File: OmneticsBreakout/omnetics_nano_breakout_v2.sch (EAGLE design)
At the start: 2 parts

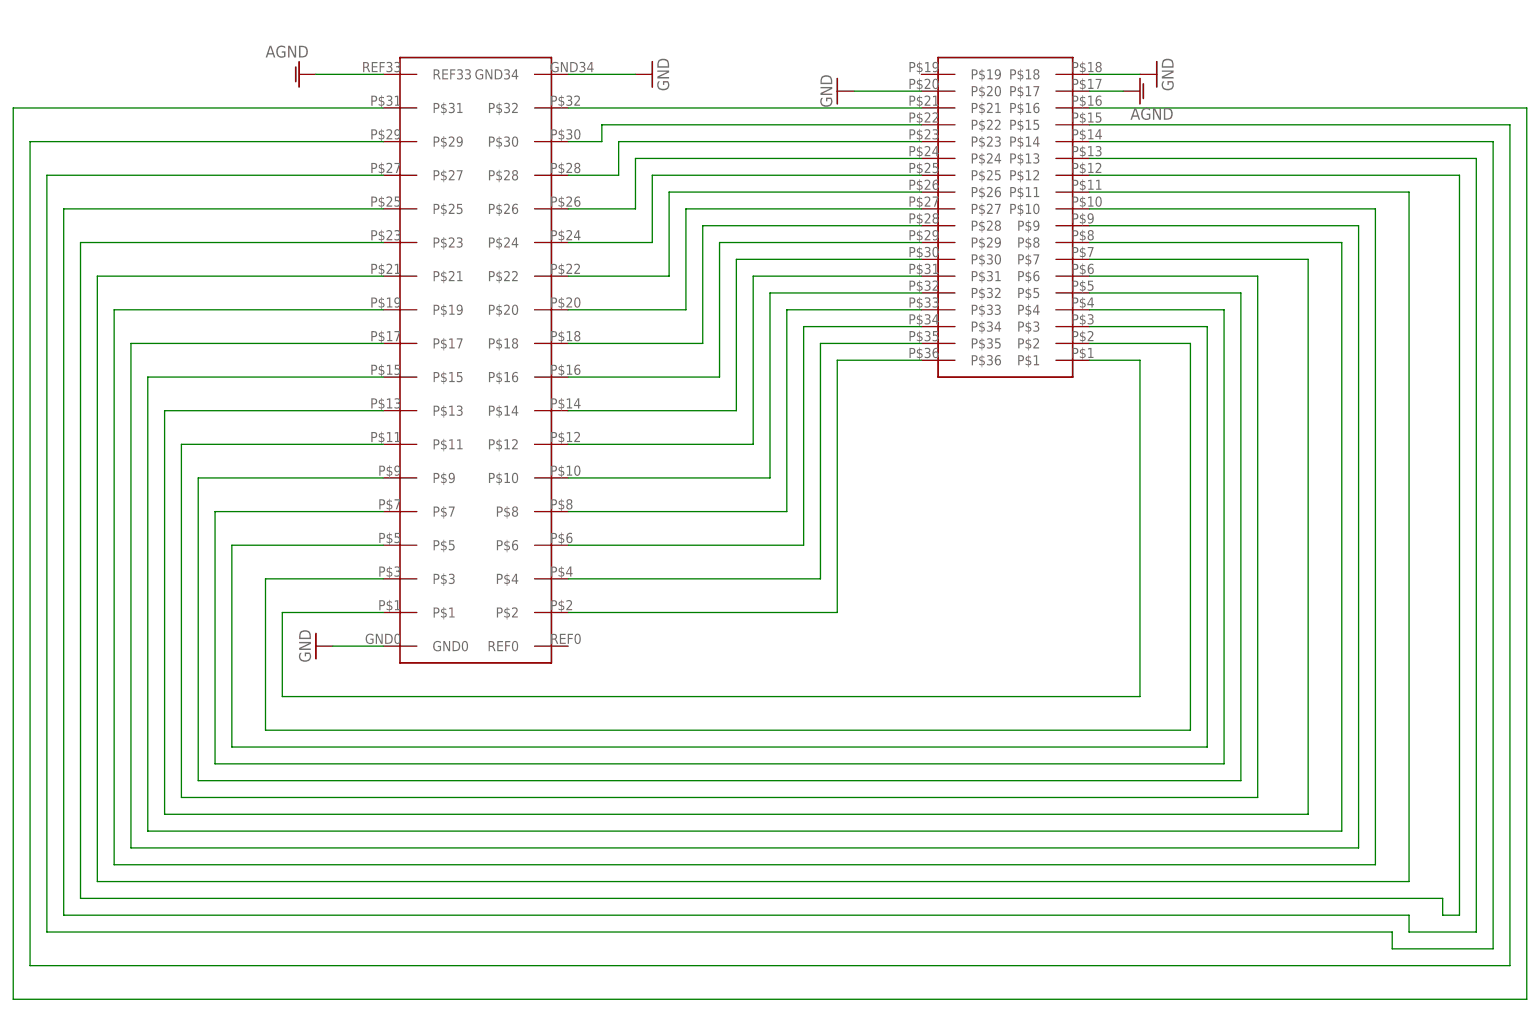
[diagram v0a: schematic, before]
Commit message: omentics breakout board
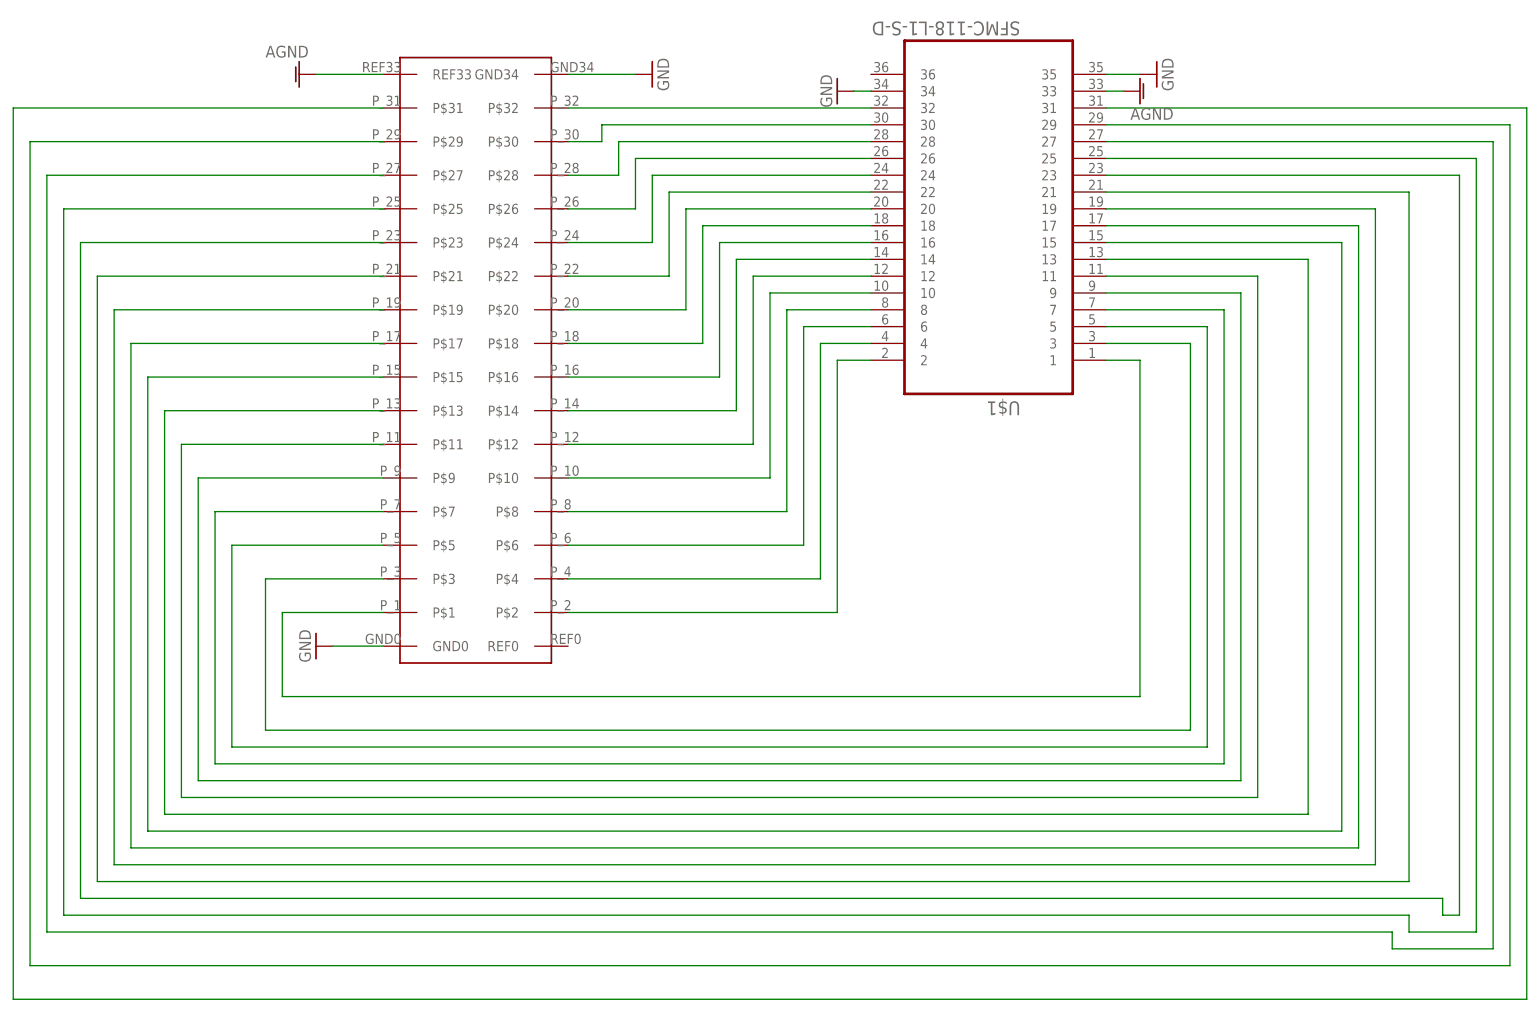
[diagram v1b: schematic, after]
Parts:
- U$1: value FSTH-118-01-F-D -> SFMC-118-L1-S-D; device Sombeck_lib:FSTH-118-01-F-D -> tuckerLib:SFMC-118-L1-S-D
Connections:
- net AGND: now also U$1.33; no longer U$1.P$17
- net GND: now also U$1.34, U$1.35; no longer U$1.P$18, U$1.P$20
- net N$1: now also U$1.1; no longer U$1.P$1
- net N$10: now also U$1.18; no longer U$1.P$28
- net N$11: now also U$1.20; no longer U$1.P$27
- net N$12: now also U$1.22; no longer U$1.P$26
- net N$13: now also U$1.24; no longer U$1.P$25
- net N$14: now also U$1.26; no longer U$1.P$24
- net N$15: now also U$1.28; no longer U$1.P$23
- net N$16: now also U$1.30; no longer U$1.P$22
- net N$17: now also U$1.32; no longer U$1.P$21
- net N$18: now also U$1.3; no longer U$1.P$2
- net N$19: now also U$1.5; no longer U$1.P$3
- net N$2: now also U$1.2; no longer U$1.P$36
- net N$20: now also U$1.7; no longer U$1.P$4
- net N$21: now also U$1.9; no longer U$1.P$5
- net N$22: now also U$1.11; no longer U$1.P$6
- net N$23: now also U$1.13; no longer U$1.P$7
- net N$24: now also U$1.15; no longer U$1.P$8
- net N$25: now also U$1.17; no longer U$1.P$9
- net N$26: now also U$1.19; no longer U$1.P$10
- net N$27: now also U$1.21; no longer U$1.P$11
- net N$28: now also U$1.23; no longer U$1.P$12
- net N$29: now also U$1.25; no longer U$1.P$13
- net N$3: now also U$1.4; no longer U$1.P$35
- net N$30: now also U$1.27; no longer U$1.P$14
- net N$31: now also U$1.29; no longer U$1.P$15
- net N$32: now also U$1.31; no longer U$1.P$16
- net N$4: now also U$1.6; no longer U$1.P$34
- net N$5: now also U$1.8; no longer U$1.P$33
- net N$6: now also U$1.10; no longer U$1.P$32
- net N$7: now also U$1.12; no longer U$1.P$31
- net N$8: now also U$1.14; no longer U$1.P$30
- net N$9: now also U$1.16; no longer U$1.P$29
